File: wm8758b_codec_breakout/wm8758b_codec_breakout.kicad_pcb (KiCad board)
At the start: 2 copper layers, 40 x 40 mm, 21 parts, among them J1 Conn_01x12, J101 AudioJack3, J102 AudioJack3, J2 Conn_01x12, U1 WM8758B

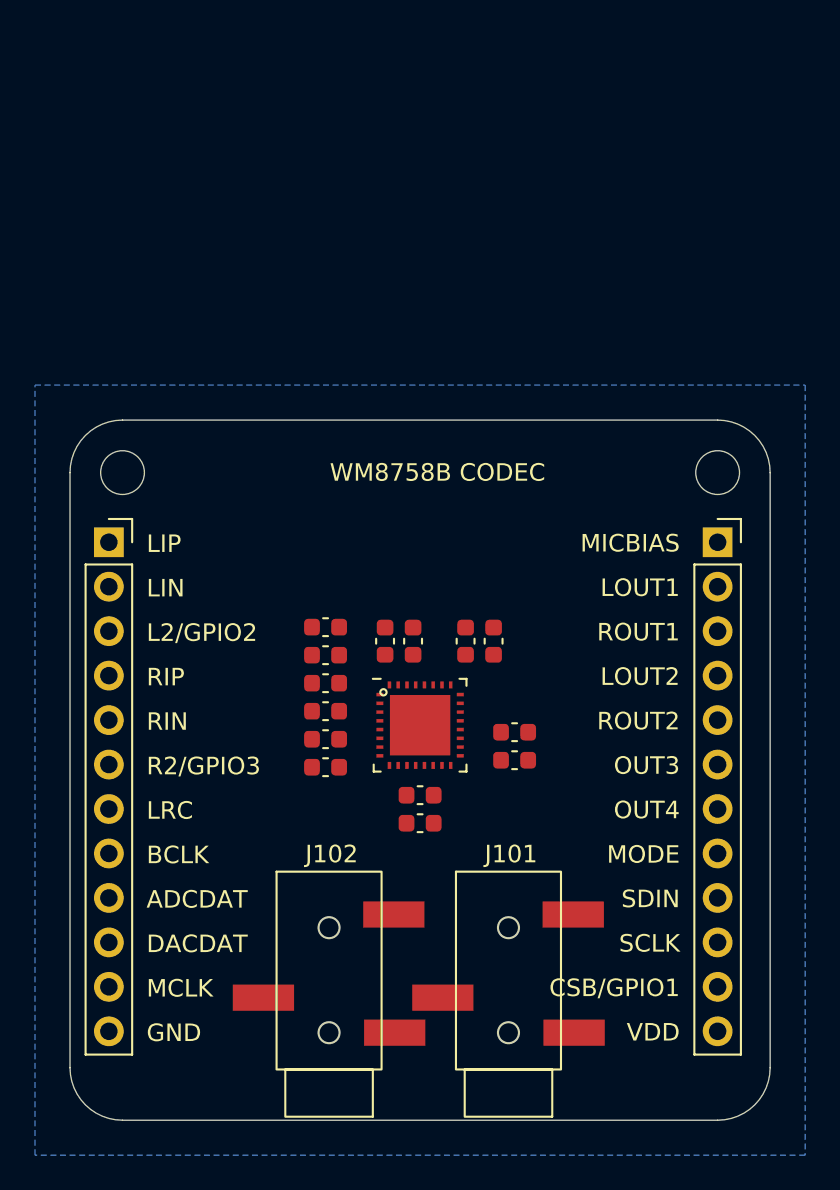
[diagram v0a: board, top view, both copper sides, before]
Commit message: WIP
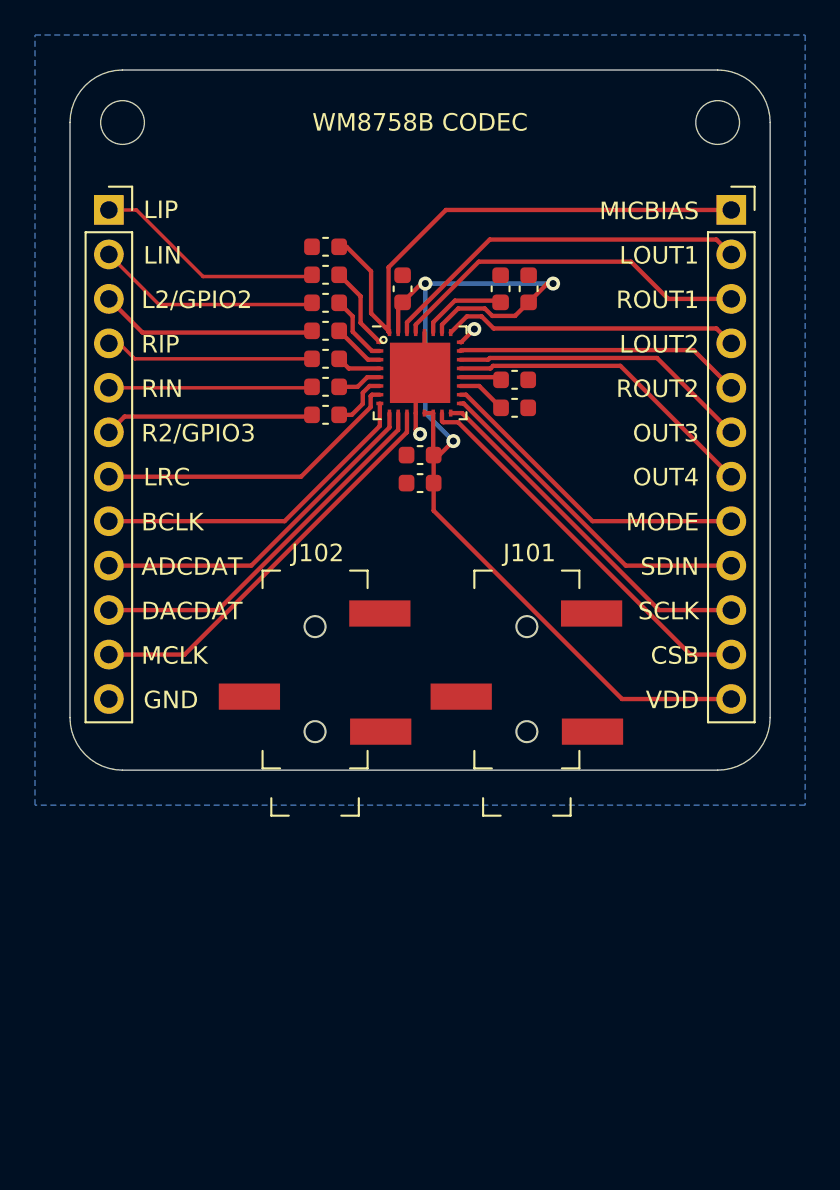
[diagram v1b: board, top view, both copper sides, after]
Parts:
- moved C6 22.8 mm to (144.6, 70.1), turned to 180 degrees
- moved C2 20.2 mm to (156.2, 72.5)
- moved C5 20.2 mm to (154.6, 72.5)
- moved C1 20.1 mm to (149.0, 72.5)
- moved C11 20.1 mm to (144.6, 78.1)
- moved C12 20.1 mm to (155.4, 79.3)
- moved C16 20.1 mm to (144.6, 73.3)
- moved U1 20.1 mm to (150.0, 77.3)
- moved C10 20.1 mm to (144.6, 74.9)
- moved C13 20.1 mm to (155.4, 77.7)
- moved C15 20.1 mm to (144.6, 71.7)
- moved C19 20.1 mm to (144.6, 76.5)
- moved C8 20.1 mm to (144.6, 79.7)
- moved REF** 20.0 mm to (167.0, 63.0)
- moved REF** 20.0 mm to (133.0, 63.0)
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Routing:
- net VDD: track 0.00 -> 57.7 mm, vias 0 -> 3
- net MICBIAS: track 0.00 -> 31.0 mm
- net MCLK: track 0.00 -> 23.4 mm
- net CSB_GPIO1: track 0.00 -> 22.5 mm
- net DACDAT: track 0.00 -> 21.8 mm
- net LOUT1: track 0.00 -> 21.4 mm
- net ROUT1: track 0.00 -> 20.9 mm
- net SCLK: track 0.00 -> 20.7 mm
- net ADCDAT: track 0.00 -> 20.1 mm
- net SDIN: track 0.00 -> 19.3 mm
- net BCLK: track 0.00 -> 19.0 mm
- net MODE: track 0.00 -> 18.5 mm
- net OUT4: track 0.00 -> 18.2 mm
- net LRC: track 0.00 -> 17.8 mm
- net OUT3: track 0.00 -> 17.3 mm
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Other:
- board text added: "CSB"
- board text added: "V1"
- board text removed: "CSB/GPIO1"
